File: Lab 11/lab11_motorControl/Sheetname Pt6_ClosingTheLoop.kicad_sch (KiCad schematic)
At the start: 1 part, among them U4 LM324

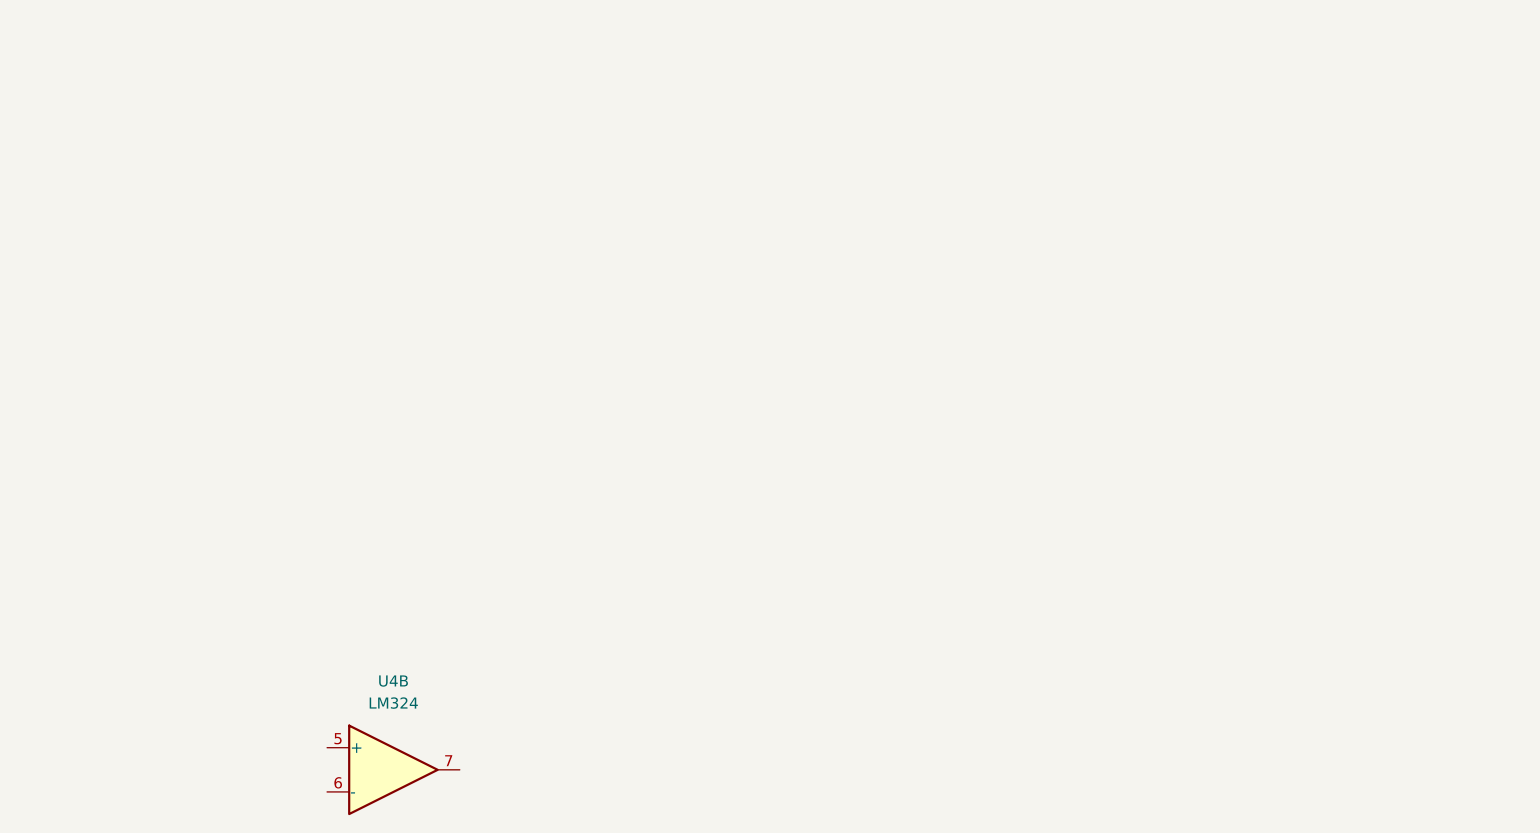
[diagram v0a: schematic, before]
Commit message: Lab 11
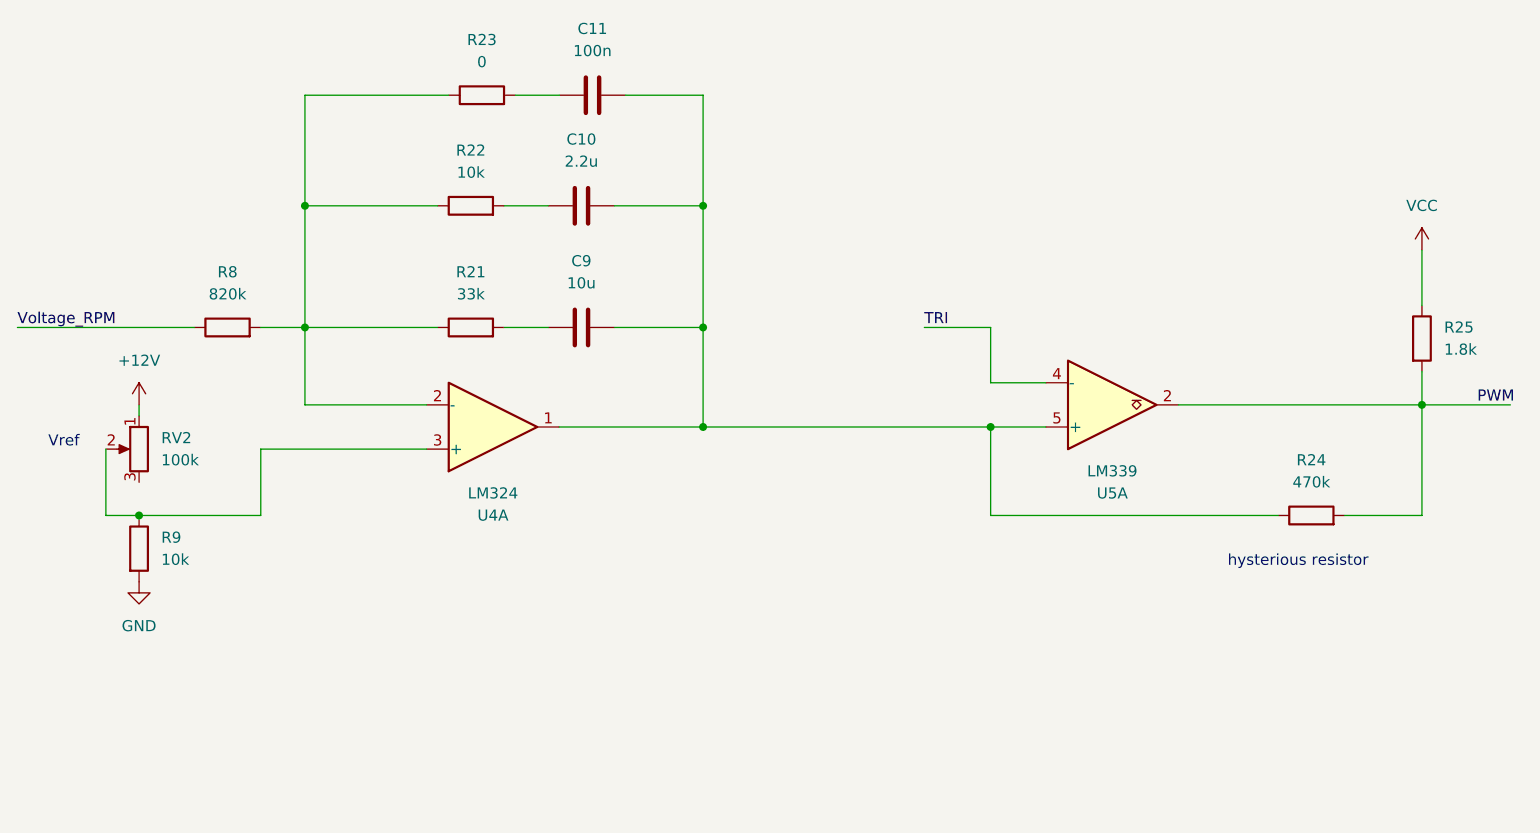
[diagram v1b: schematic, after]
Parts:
- removed U4: LM324, symbol Amplifier_Operational:LM324
- added C10: 2.2u, symbol Device:C
- added C11: 100n, symbol Device:C
- added C9: 10u, symbol Device:C
- added R21: 33k, symbol Device:R
- added R22, R9: 10k, symbol Device:R
- added R23: 0, symbol Device:R
- added R24: 470k, symbol Device:R
- added R25: 1.8k, symbol Device:R
- added R8: 820k, symbol Device:R
- added RV2: 100k, symbol Device:R_Potentiometer
- added U4: LM324, symbol Amplifier_Operational:LM324
- added U5: LM339, symbol Comparator:LM339
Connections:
- new net: C10.2, C11.2, C9.2, R24.1, U4.1, U5.5 (+)
- new net: R9.1, RV2.2, U4.3 (+)
- new net: R21.1, R22.1, R23.1, R8.2, U4.2 (-)
- new net: C11.1, R23.2
- new net: C10.1, R22.2
- new net: C9.1, R21.2
- new net +12V: RV2.1
- new net GND: R9.2
- new net PWM: R24.2, R25.2, U5.2
- new net TRI: U5.4 (-)
- new net VCC: R25.1
- new net Voltage_RPM: R8.1
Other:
- note added: "Vref"
- note added: "hysterious resistor"
